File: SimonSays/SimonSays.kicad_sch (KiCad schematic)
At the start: 22 parts, among them SW1 SW_Push, SW2 SW_Push, SW3 SW_Push, SW4 SW_Push, X1 Crystal

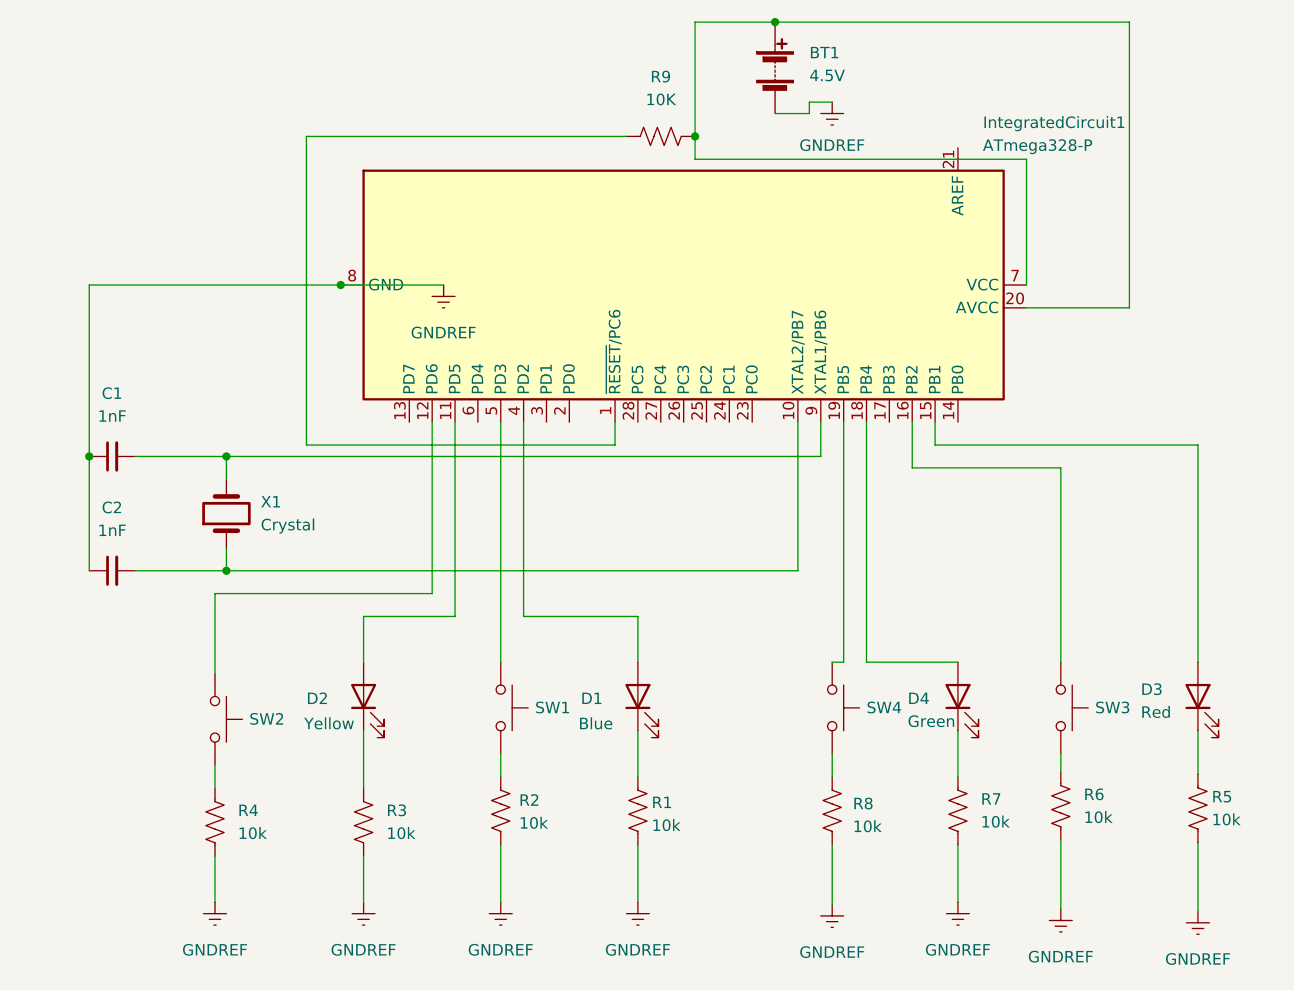
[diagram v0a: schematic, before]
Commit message: Added
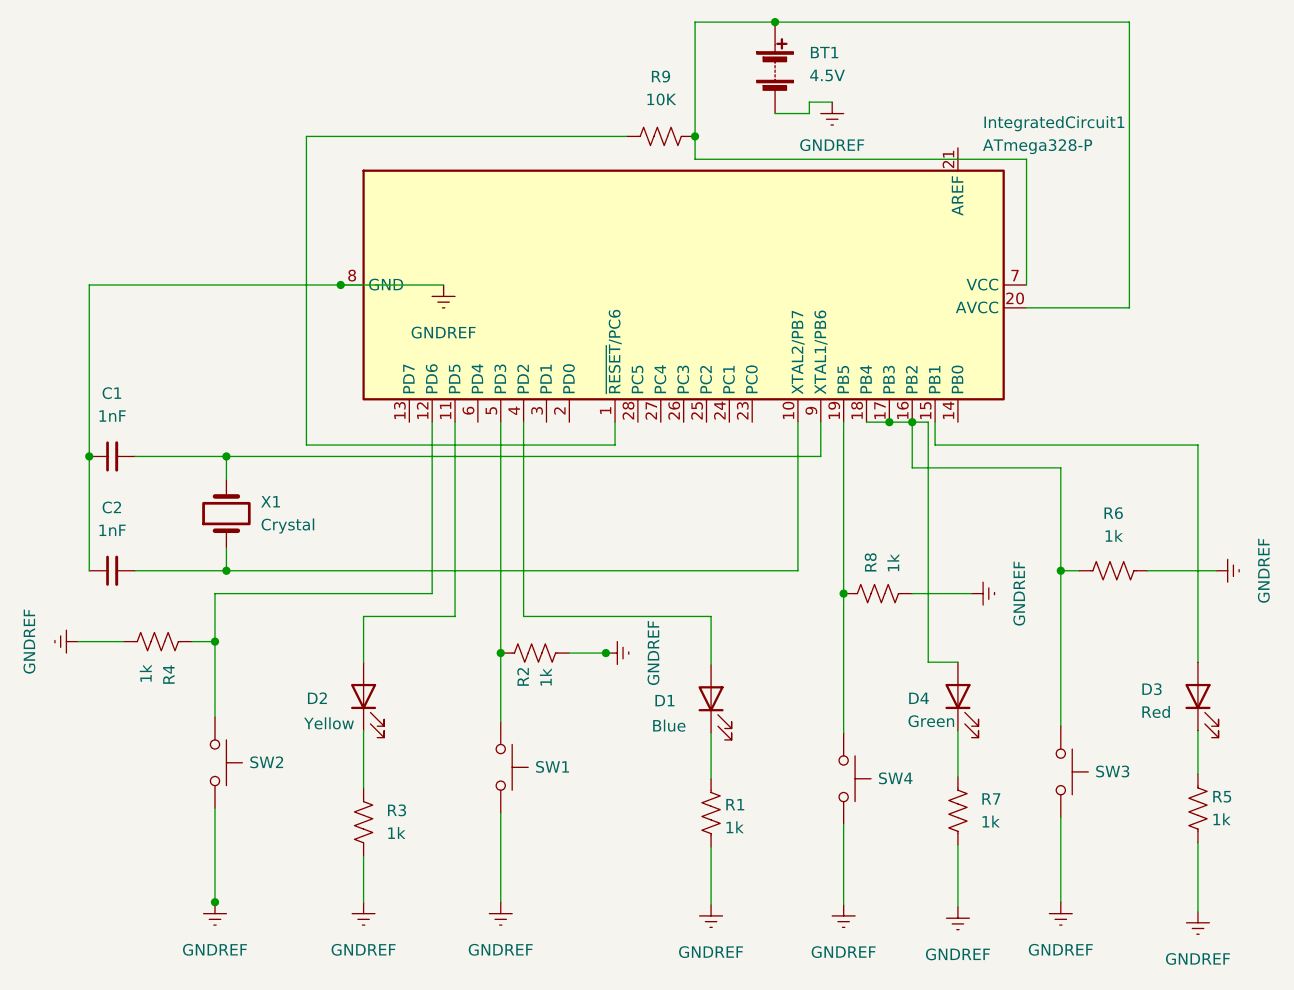
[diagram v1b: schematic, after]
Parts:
- BT1: footprint Battery:BatteryHolder_Keystone_2479_3xAAA -> Battery:BatteryHolder_ComfortableElectronic_CH273-2450_1x2450
- R1, R2, R3, R4, R5, R6, R7, R8: value 10k -> 1k
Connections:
- net GNDREF: now also SW1.2, SW2.2, SW3.2, SW4.2
- net at R4.1: now also IntegratedCircuit1.12 (PD6), SW2.1; no longer SW2.2
- net at R2.1: now also IntegratedCircuit1.5 (PD3), SW1.1; no longer SW1.2
- net at R8.1: now also IntegratedCircuit1.19 (PB5), SW4.1; no longer SW4.2
- net at IntegratedCircuit1.16 (PB2), SW3.1: now also D4.2 (A), IntegratedCircuit1.17 (PB3), IntegratedCircuit1.18 (PB4), R6.1
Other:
- moved on the sheet: SW1, SW2, SW3, SW4
